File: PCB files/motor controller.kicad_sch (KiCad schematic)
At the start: 37 parts, among them J1 ISP, J10 5V, J11 5V, J2 I2C, J3 Motor Signal, J4 M1, J5 M2, J6 RST_Jump, J7 RST_Jump, J8 GND, J9 5V, SW1 reset, U1 ATmega328-P, Y1 16Mhz

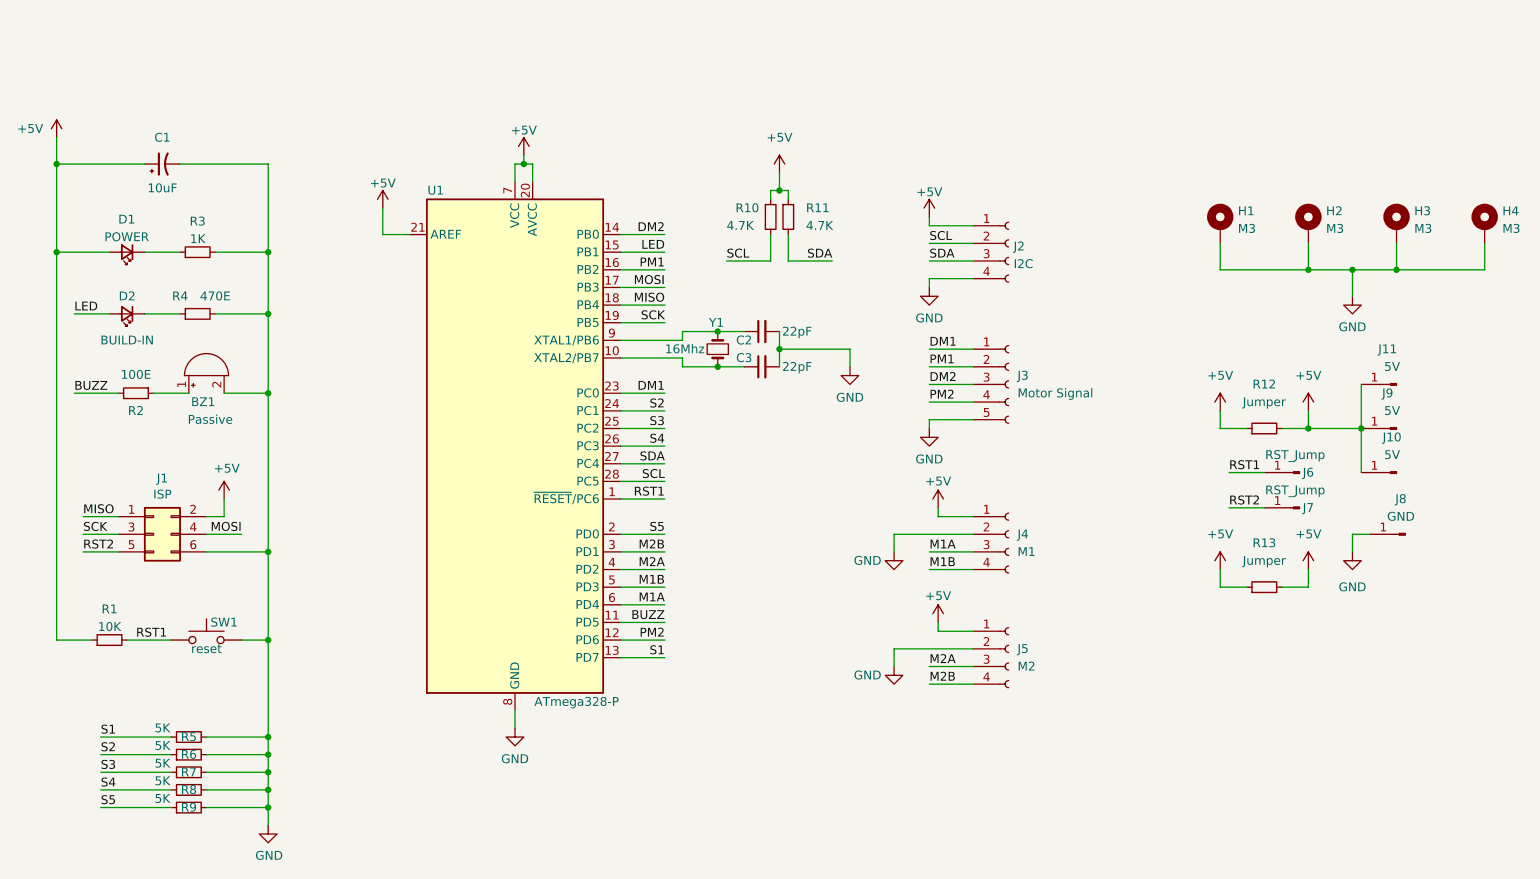
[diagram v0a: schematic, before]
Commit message: backups
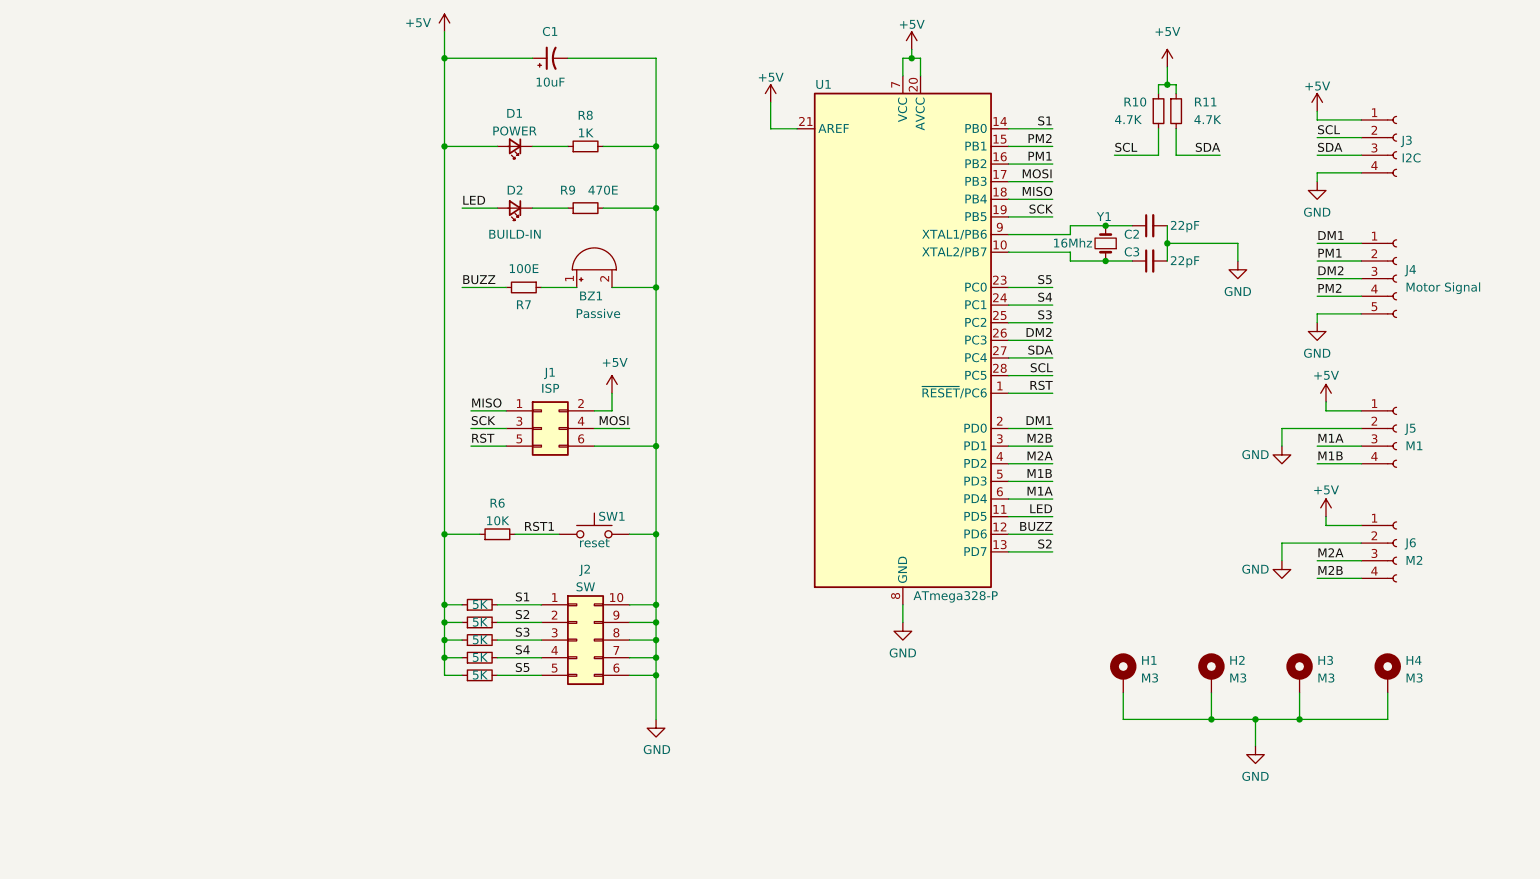
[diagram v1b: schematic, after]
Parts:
- removed J10, J11, J9: 5V, Connector_PinHeader_2.54mm:PinHeader_1x01_P2.54mm_Vertical, symbol Connector:Conn_01x01_Male
- removed J6, J7: RST_Jump, Connector_PinHeader_2.54mm:PinHeader_1x01_P2.54mm_Vertical, symbol Connector:Conn_01x01_Male
- removed J8: GND, Connector_PinHeader_2.54mm:PinHeader_1x01_P2.54mm_Vertical, symbol Connector:Conn_01x01_Male
- removed R12: Jumper, Resistor_THT:R_Axial_DIN0207_L6.3mm_D2.5mm_P7.62mm_Horizontal, symbol Device:R_Small
- removed R13: Jumper, Resistor_THT:R_Axial_DIN0207_L6.3mm_D2.5mm_P10.16mm_Horizontal, symbol Device:R_Small
- removed R6, R7, R8, R9: 5K, Resistor_THT:R_Axial_DIN0204_L3.6mm_D1.6mm_P2.54mm_Vertical, symbol Device:R_Small
- added J2: SW, Button_Switch_THT:SW_DIP_SPSTx05_Slide_9.78x14.88mm_W7.62mm_P2.54mm, symbol Connector_Generic:Conn_02x05_Counter_Clockwise
- added R1, R2, R3, R4: 5K, Resistor_SMD:R_0805_2012Metric, symbol Device:R_Small
- C1: footprint Capacitor_THT:CP_Radial_D4.0mm_P2.00mm -> Capacitor_SMD:CP_Elec_6.3x4.5
- C2, C3: footprint Capacitor_THT:C_Disc_D3.4mm_W2.1mm_P2.50mm -> Capacitor_SMD:C_0805_2012Metric
- D1, D2: footprint LED_THT:LED_D3.0mm -> LED_SMD:LED_0805_2012Metric
- R10, R11: footprint Resistor_THT:R_Axial_DIN0207_L6.3mm_D2.5mm_P7.62mm_Horizontal -> Resistor_SMD:R_0805_2012Metric
- R5: footprint Resistor_THT:R_Axial_DIN0204_L3.6mm_D1.6mm_P5.08mm_Horizontal -> Resistor_SMD:R_0805_2012Metric
- R6: renamed from R1; footprint Resistor_THT:R_Axial_DIN0207_L6.3mm_D2.5mm_P7.62mm_Horizontal -> Resistor_SMD:R_0805_2012Metric
- R7: renamed from R2; footprint Resistor_THT:R_Axial_DIN0207_L6.3mm_D2.5mm_P7.62mm_Horizontal -> Resistor_SMD:R_0805_2012Metric
- R8: renamed from R3; footprint Resistor_THT:R_Axial_DIN0207_L6.3mm_D2.5mm_P7.62mm_Horizontal -> Resistor_SMD:R_0805_2012Metric
- R9: renamed from R4; footprint Resistor_THT:R_Axial_DIN0207_L6.3mm_D2.5mm_P7.62mm_Horizontal -> Resistor_SMD:R_0805_2012Metric
- Y1: footprint Crystal:Crystal_HC49-4H_Vertical -> Crystal:Crystal_SMD_HC49-SD
- renumbered J2 to J3, J3 to J4, J4 to J5, J5 to J6
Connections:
- net +5V: now also R5.1, R1.1, R2.1, R3.1, R4.1
- net BUZZ: now also U1.12 (PD6); no longer U1.11 (PD5)
- net DM1: now also U1.2 (PD0); no longer U1.23 (PC0)
- net DM2: now also U1.26 (PC3); no longer U1.14 (PB0)
- net GND: now also J2.10 (Pin_10), J2.6 (Pin_6), J2.7 (Pin_7), J2.8 (Pin_8), J2.9 (Pin_9); no longer R5.2
- net LED: now also U1.11 (PD5); no longer U1.15 (PB1)
- net PM2: now also U1.15 (PB1); no longer U1.12 (PD6)
- net RST1: no longer U1.1 (~{RESET}/PC6)
- net S1: now also U1.14 (PB0), J2.1 (Pin_1), R1.2; no longer R5.1, U1.13 (PD7)
- net S2: now also U1.13 (PD7), J2.2 (Pin_2), R2.2; no longer U1.24 (PC1)
- net S3: now also J2.3 (Pin_3), R3.2
- net S4: now also U1.24 (PC1), J2.4 (Pin_4), R4.2; no longer U1.26 (PC3)
- net S5: now also R5.2, U1.23 (PC0), J2.5 (Pin_5); no longer U1.2 (PD0)
- net RST2 renamed RST
- net RST: now also U1.1 (~{RESET}/PC6)
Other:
- moved on the sheet: BZ1, C1, C2, C3, D1, D2, H1, H2, H3, H4, J1, J3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

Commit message: updated track width
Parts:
- C1: footprint Capacitor_SMD:CP_Elec_6.3x4.5 -> Capacitor_SMD:CP_Elec_4x3.9
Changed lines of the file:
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@@
       (effects (font (size 1.27 1.27)))
     )
-    (property "Footprint" "Capacitor_SMD:CP_Elec_6.3x4.5" (at 93.98 41.91 0)
+    (property "Footprint" "Capacitor_SMD:CP_Elec_4x3.9" (at 93.98 41.91 0)
       (effects (font (size 1.27 1.27)) hide)
     )
